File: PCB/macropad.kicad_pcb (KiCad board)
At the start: 2 copper layers, 83.5 x 97.3 mm, 40 parts, among them SW1 Kailh Choc V2, SW10 Kailh Choc V2, SW11 Kailh Choc V2, SW12 Kailh Choc V2, SW13 Kailh Choc V2, SW14 Kailh Choc V2, SW15 Kailh Choc V2, SW16 Kailh Choc V2, SW2 Kailh Choc V2, SW3 Kailh Choc V2, SW4 Kailh Choc V2, SW5 Kailh Choc V2, SW6 Kailh Choc V2, SW7 Kailh Choc V2, SW8 Kailh Choc V2, SW9 Kailh Choc V2, U2 SEEEDUINO XIAO RP2040

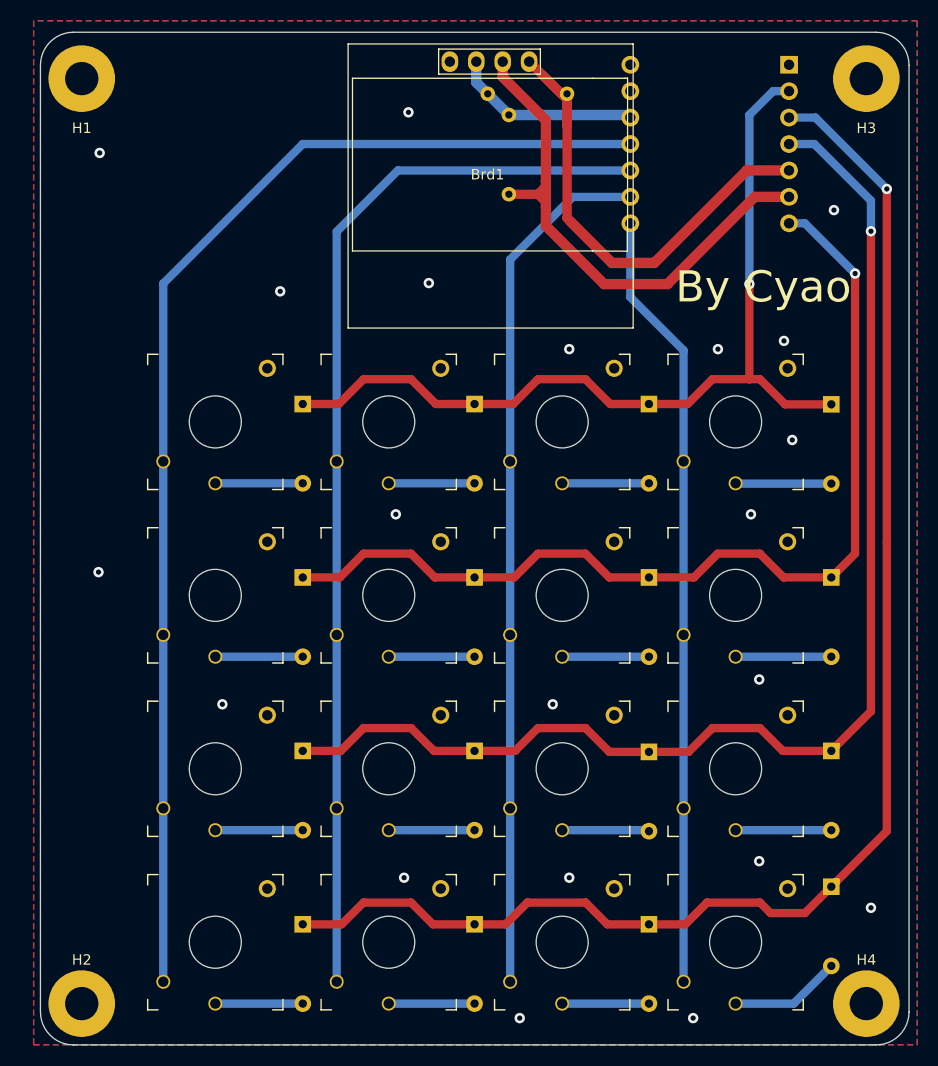
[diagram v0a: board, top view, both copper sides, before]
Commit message: Redisigned PCB
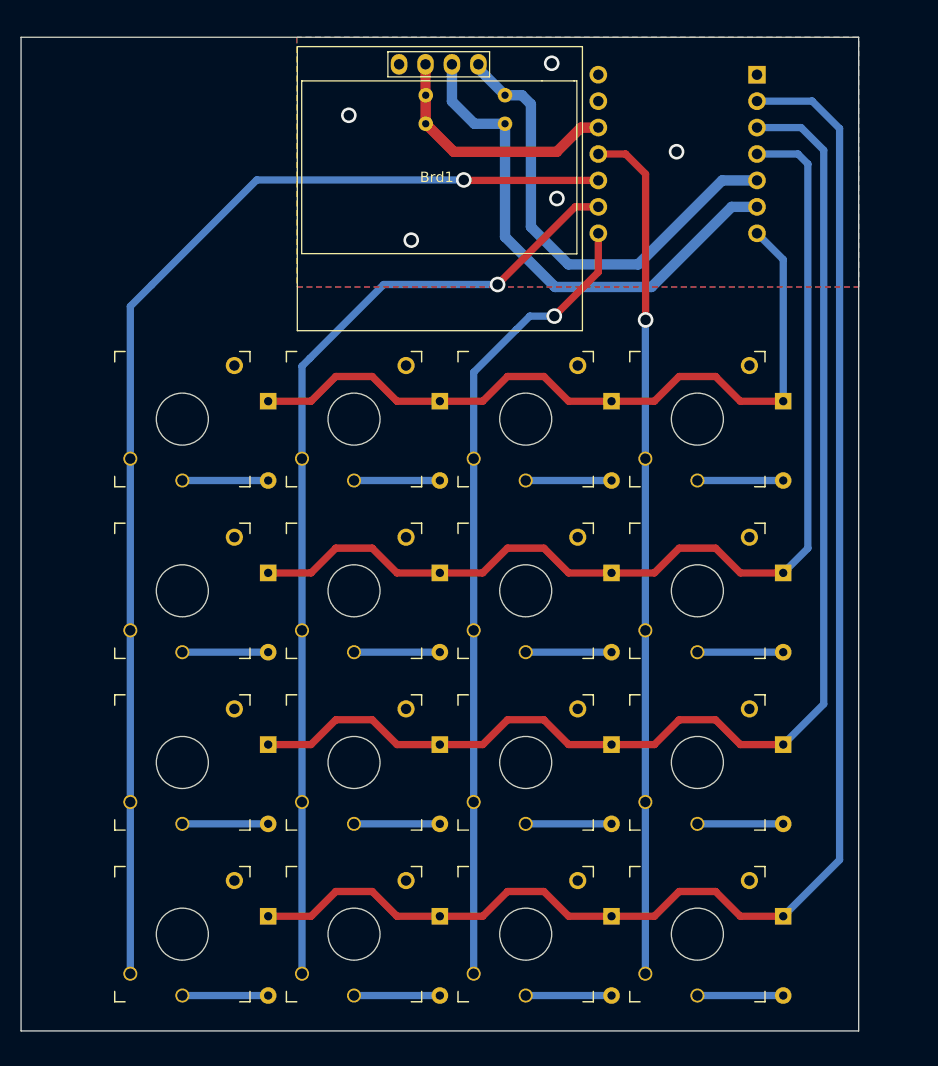
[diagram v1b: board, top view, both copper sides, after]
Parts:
- removed H1, H2, H3, H4: Mounting Hole, MountingHole:MountingHole_3.2mm_M3_Pad
- R1, R2: value Resistor 4.7k ohm -> 4.7k
- moved R1 8.04 mm to (143.4, 58.3), turned to 0 degrees
- moved R2 5.96 mm to (143.4, 55.6)
- moved D13 5.43 mm to (177.8, 134.5)
- moved Brd1 4.89 mm to (144.4, 63.2)
- moved D12 4.66 mm to (177.8, 118.0)
- moved D11 4.64 mm to (177.8, 101.5)
- moved D10 4.63 mm to (177.8, 85.0)
- moved SW13 3.75 mm to (169.5, 136.2)
- moved SW12 3.72 mm to (169.5, 119.7)
- moved SW11 3.70 mm to (169.5, 103.2)
- moved SW10 3.68 mm to (169.5, 86.7)
- moved D14 3.68 mm to (161.2, 134.5)
- moved D9 3.66 mm to (161.2, 118.0)
- moved D6 3.62 mm to (161.2, 101.5)
- moved D3 3.61 mm to (161.2, 85.0)
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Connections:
- U2 pad 10: COL1 -> COL0
- U2 pad 11: COL0 -> COL3
- U2 pad 2: ROW0 -> ROW3
- U2 pad 3: ROW3 -> ROW2
- U2 pad 4: ROW2 -> ROW1
- U2 pad 7: ROW1 -> ROW0
- U2 pad 8: COL3 -> COL2
- U2 pad 9: COL2 -> COL1
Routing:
- net ROW0: track 87.0 -> 72.6 mm, vias 1 -> 0
- net COL1: track 102.8 -> 93.2 mm, vias 0 -> 1
- net COL3: track 75.0 -> 82.6 mm, vias 0 -> 1
- net ROW1: track 95.0 -> 101.4 mm, vias 1 -> 0
- net +3.3V: track 18.2 -> 24.5 mm
- net COL2: track 83.5 -> 77.5 mm, vias 0 -> 1
- net Net-(Brd1-SDA): track 49.5 -> 45.2 mm
- net ROW3: track 138.1 -> 142.4 mm, vias 1 -> 0
- net COL0: track 117.6 -> 114.2 mm, vias 0 -> 1
- net Net-(Brd1-SCL): track 52.5 -> 49.8 mm
- net Net-(D13-A): track 10.7 -> 8.25 mm
- net Net-(D10-A): track 9.21 -> 8.25 mm
- net Net-(D12-A): track 9.20 -> 8.25 mm
- net Net-(D11-A): track 9.20 -> 8.25 mm
- net ROW2: track 120.9 -> 121.5 mm, vias 1 -> 0
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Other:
- board size 83.5 x 97.3 mm -> 80.5 x 95.5 mm
- board text added: "Cyaopad"
- board text added: "Rev 4.0"
- board text removed: "By Cyao"
